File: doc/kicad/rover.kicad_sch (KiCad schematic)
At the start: 10 parts, among them J1 I2C, J2 UART, J3 UART, M1 DC_Motor_Enc_5pin, M2 DC_Motor_Enc_5pin, M3 DC_Motor_Enc_5pin, M4 DC_Motor_Enc_5pin, U1 STM32F411_BlackPill, U2 ESP32_C3, U3 LSM303DLHC

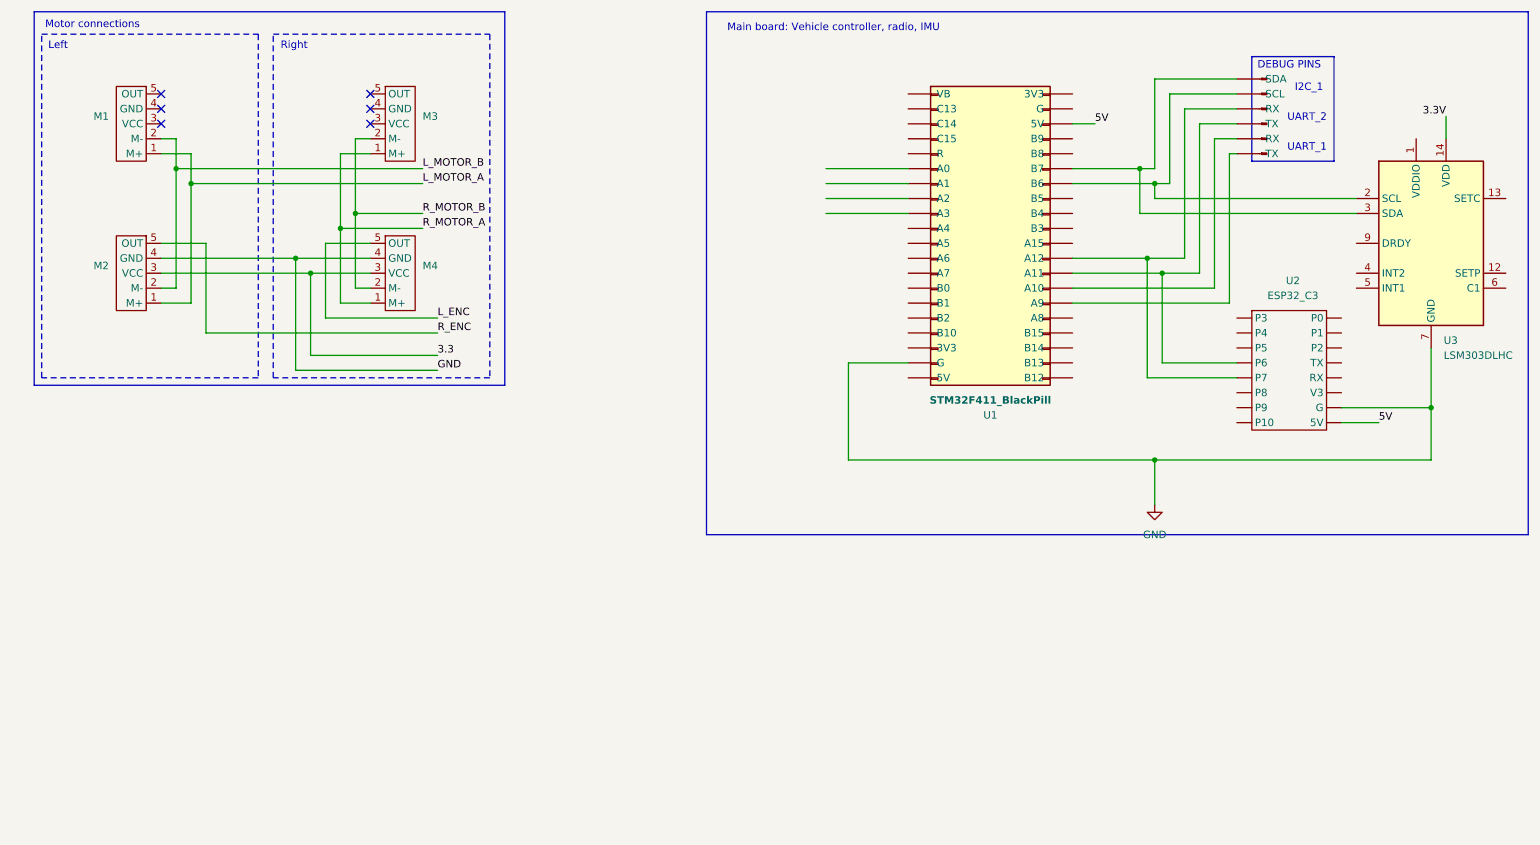
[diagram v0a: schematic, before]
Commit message: Improve motor control
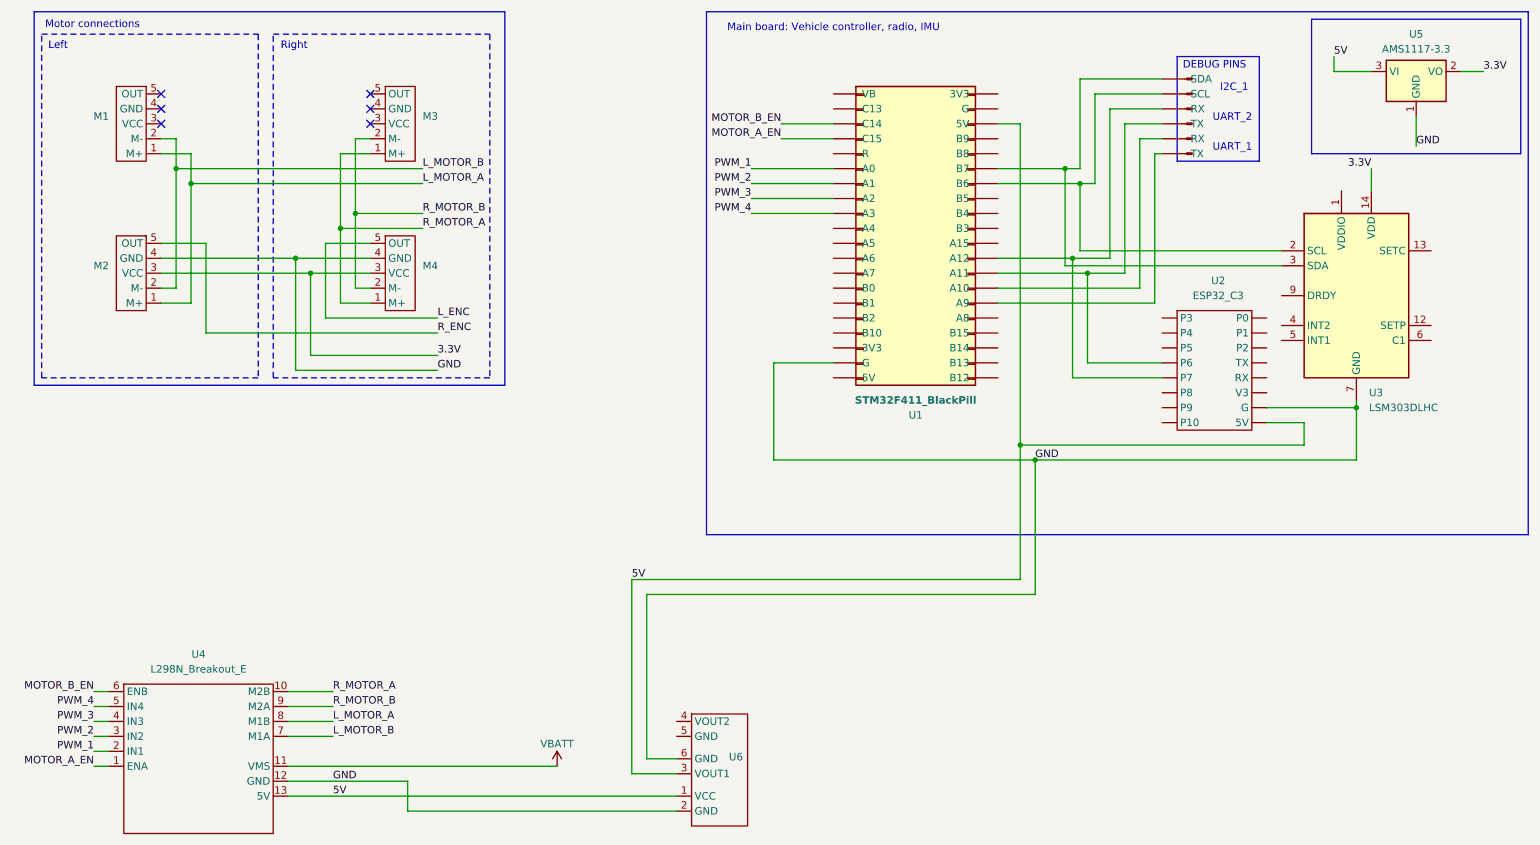
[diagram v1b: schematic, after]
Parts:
- added U4: L298N_Breakout_E, symbol DRX:L298N_Breakout_Expanded
- added U5: AMS1117-3.3, Package_TO_SOT_SMD:SOT-223-3_TabPin2, symbol Regulator_Linear:AMS1117-3.3
- added U6: ~, symbol DRX:Rover_PowerBus1
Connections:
- net 3.3 is gone; now on net 3.3V: M2.3 (VCC), M4.3 (VCC)
- net 3.3V: now also U5.2 (VO)
- net 5V: now also U4.13 (5V), U5.3 (VI), U6.1 (VCC), U6.3 (VOUT1)
- net GND: now also U4.12 (GND), U5.1 (GND), U6.2 (GND), U6.6 (GND)
- net L_MOTOR_A: now also U4.8 (M1B)
- net L_MOTOR_B: now also U4.7 (M1A)
- net R_MOTOR_A: now also U4.10 (M2B)
- net R_MOTOR_B: now also U4.9 (M2A)
- net MOTOR_B_EN: now reaches U1.3 (C14)
- net MOTOR_B_EN: now also U4.6 (ENB)
- net MOTOR_A_EN: now reaches U1.4 (C15)
- net MOTOR_A_EN: now also U4.1 (ENA)
- net PWM_1: now reaches U1.6 (A0)
- net PWM_1: now also U4.2 (IN1)
- net PWM_2: now reaches U1.7 (A1)
- net PWM_2: now also U4.3 (IN2)
- net PWM_3: now reaches U1.8 (A2)
- net PWM_3: now also U4.4 (IN3)
- net PWM_4: now reaches U1.9 (A3)
- net PWM_4: now also U4.5 (IN4)
- new net VBATT: U4.11 (VMS)
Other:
- moved on the sheet: U1, U2, U3
